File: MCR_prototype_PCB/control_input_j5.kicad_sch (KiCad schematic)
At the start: 34 parts, among them J5 Conn_01x23_Pin, U3 74AHC165

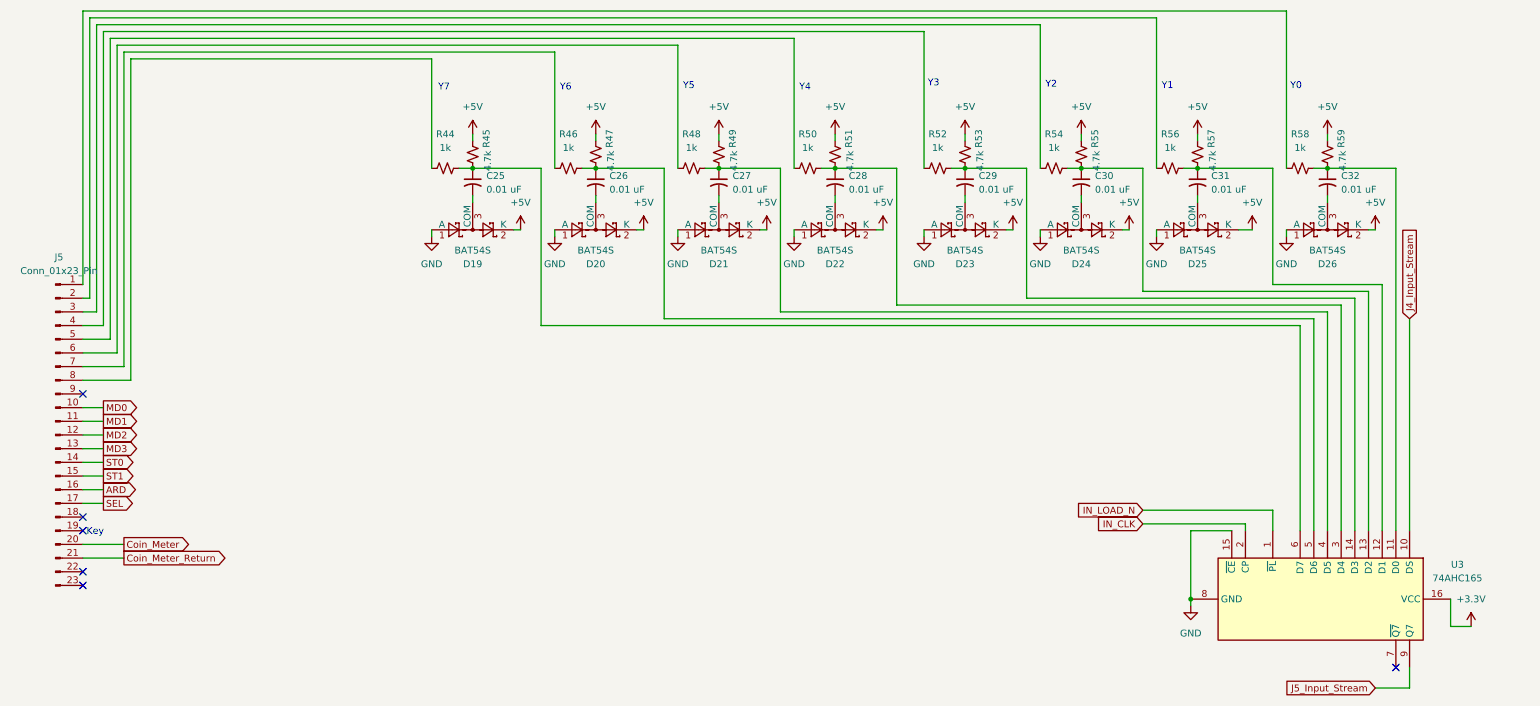
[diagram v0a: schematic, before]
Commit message: Updated 8/22/26
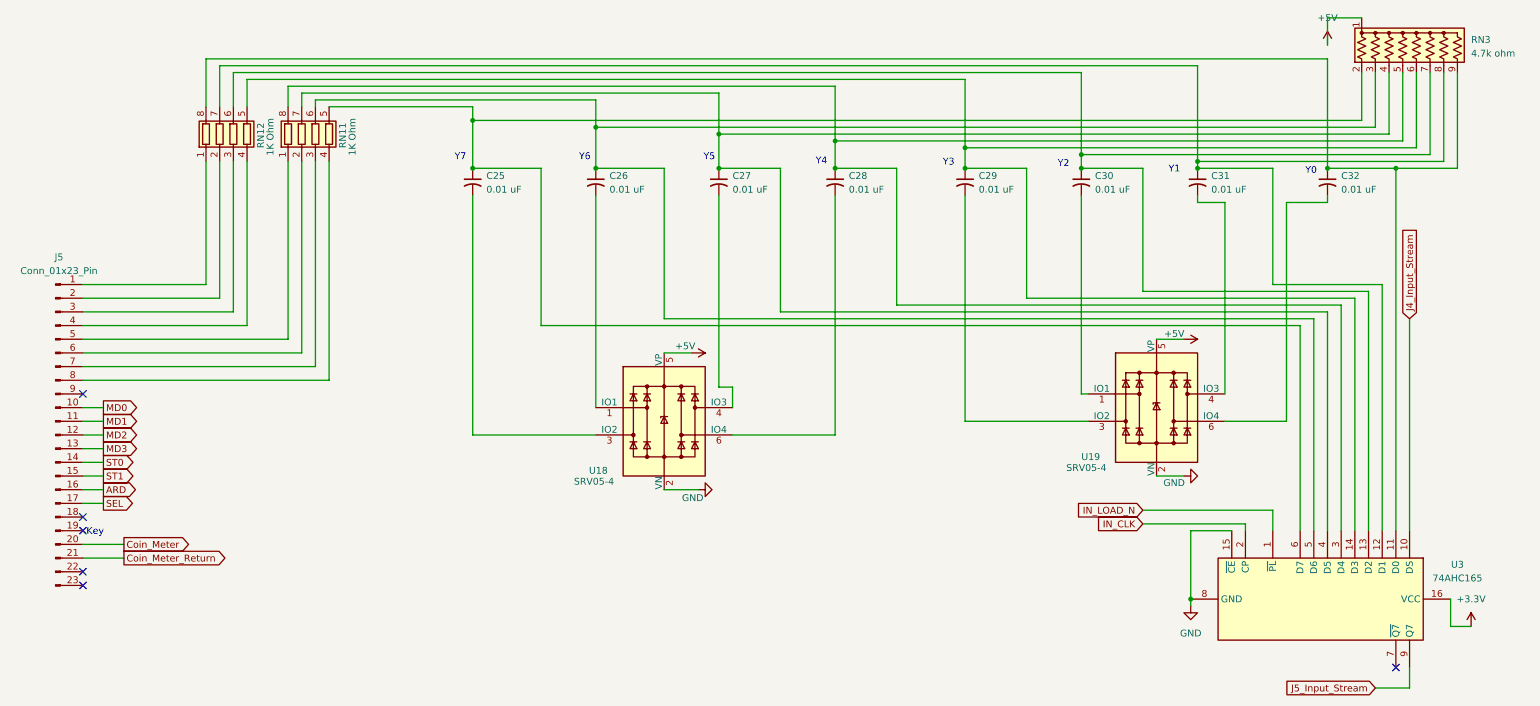
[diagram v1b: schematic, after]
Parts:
- removed D19, D20, D21, D22, D23, D24, D25, D26: BAT54S, Package_TO_SOT_SMD:SOT-23, symbol Diode:BAT54S
- removed R44, R46, R48, R50, R52, R54, R56, R58: 1k, Resistor_SMD:R_0805_2012Metric, symbol Device:R_Small_US
- removed R45, R47, R49, R51, R53, R55, R57, R59: 4.7k, Resistor_SMD:R_0805_2012Metric, symbol Device:R_Small_US
- added RN11, RN12: 1K Ohm, Resistor_SMD:R_Array_Convex_4x0603, symbol Device:R_Pack04
- added RN3: 4.7k ohm, Resistor_THT:R_Array_SIP9, symbol Device:R_Network08_US
- added U18, U19: SRV05-4, Package_TO_SOT_SMD:SOT-23-6, symbol Power_Protection:SRV05-4
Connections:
- net +5V: now also RN3.1 (common), U18.5 (VP), U19.5 (VP)
- net GND: now also U18.2 (VN), U19.2 (VN)
- net at C28.1, U3.3 (D4): now also RN11.8 (R1.2), RN3.5 (R4)
- net at C28.2: now also U18.6 (IO4)
- net at C25.1, U3.6 (D7): now also RN11.5 (R4.2), RN3.2 (R1)
- net at C25.2: now also U18.3 (IO2)
- net at C26.1, U3.5 (D6): now also RN11.6 (R3.2), RN3.3 (R2)
- net at C29.1, U3.14 (D3): now also RN12.5 (R4.2), RN3.6 (R5)
- net at C29.2: now also U19.3 (IO2)
- net at C32.2: now also U19.6 (IO4)
- net at C31.1, U3.12 (D1): now also RN12.7 (R2.2), RN3.8 (R7)
- net at C31.2: now also U19.4 (IO3)
- net at C27.2: now also U18.4 (IO3)
- net at C26.2: now also U18.1 (IO1)
- net at J5.2 (Pin_2): now also RN12.2 (R2.1)
- net at C32.1, U3.11 (D0): now also RN12.8 (R1.2), RN3.9 (R8)
- net at C27.1, U3.4 (D5): now also RN11.7 (R2.2), RN3.4 (R3)
- net at J5.6 (Pin_6): now also RN11.2 (R2.1)
- net at C30.2: now also U19.1 (IO1)
- net at C30.1, U3.13 (D2): now also RN12.6 (R3.2), RN3.7 (R6)
- net at J5.3 (Pin_3): now also RN12.3 (R3.1)
- net at J5.1 (Pin_1): now also RN12.1 (R1.1)
- net at J5.4 (Pin_4): now also RN12.4 (R4.1)
- net at J5.7 (Pin_7): now also RN11.3 (R3.1)
- net at J5.8 (Pin_8): now also RN11.4 (R4.1)
- net at J5.5 (Pin_5): now also RN11.1 (R1.1)
